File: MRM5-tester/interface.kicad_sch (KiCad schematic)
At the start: 28 parts, among them J1 Conn_01x02, J2 Conn_01x02, J3 GSB1C41110SSHR, J4 PINHD_1x2_Female, J5 PINHD_1x2_Female, J6 Conn_01x05, J7 Conn_01x05, Q5 SMMBT3906LT3G, Q6 SMMBT3906LT3G, U1 CP2102N-A02-GQFN20

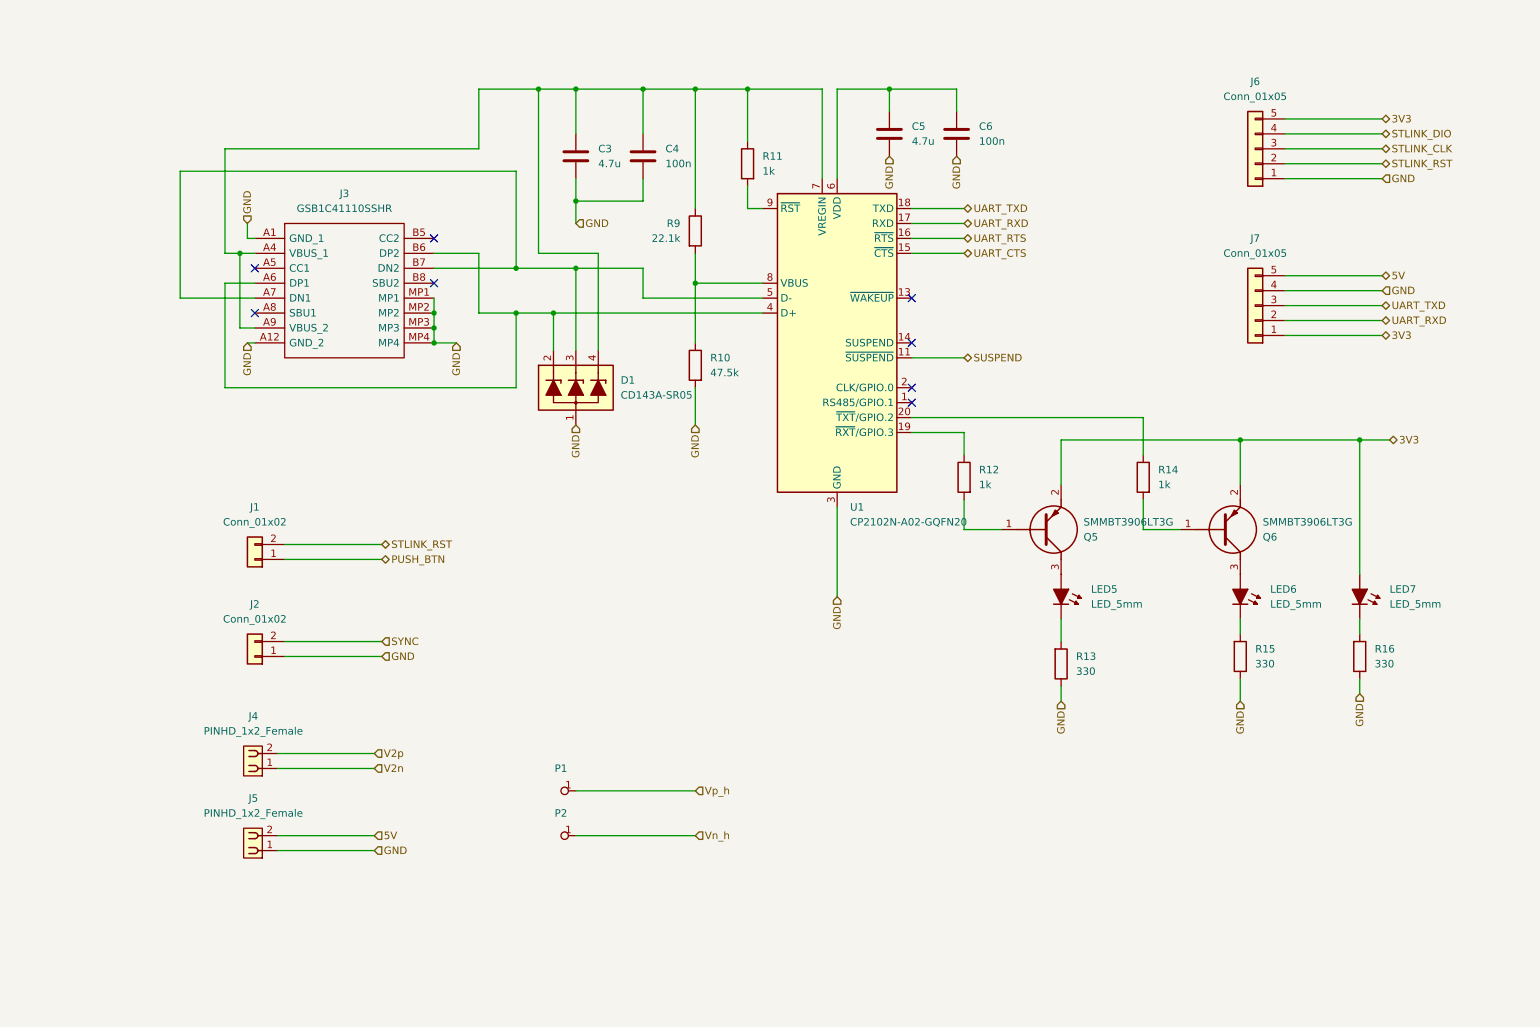
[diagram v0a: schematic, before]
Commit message: 케이스에 마춰서 제작 중
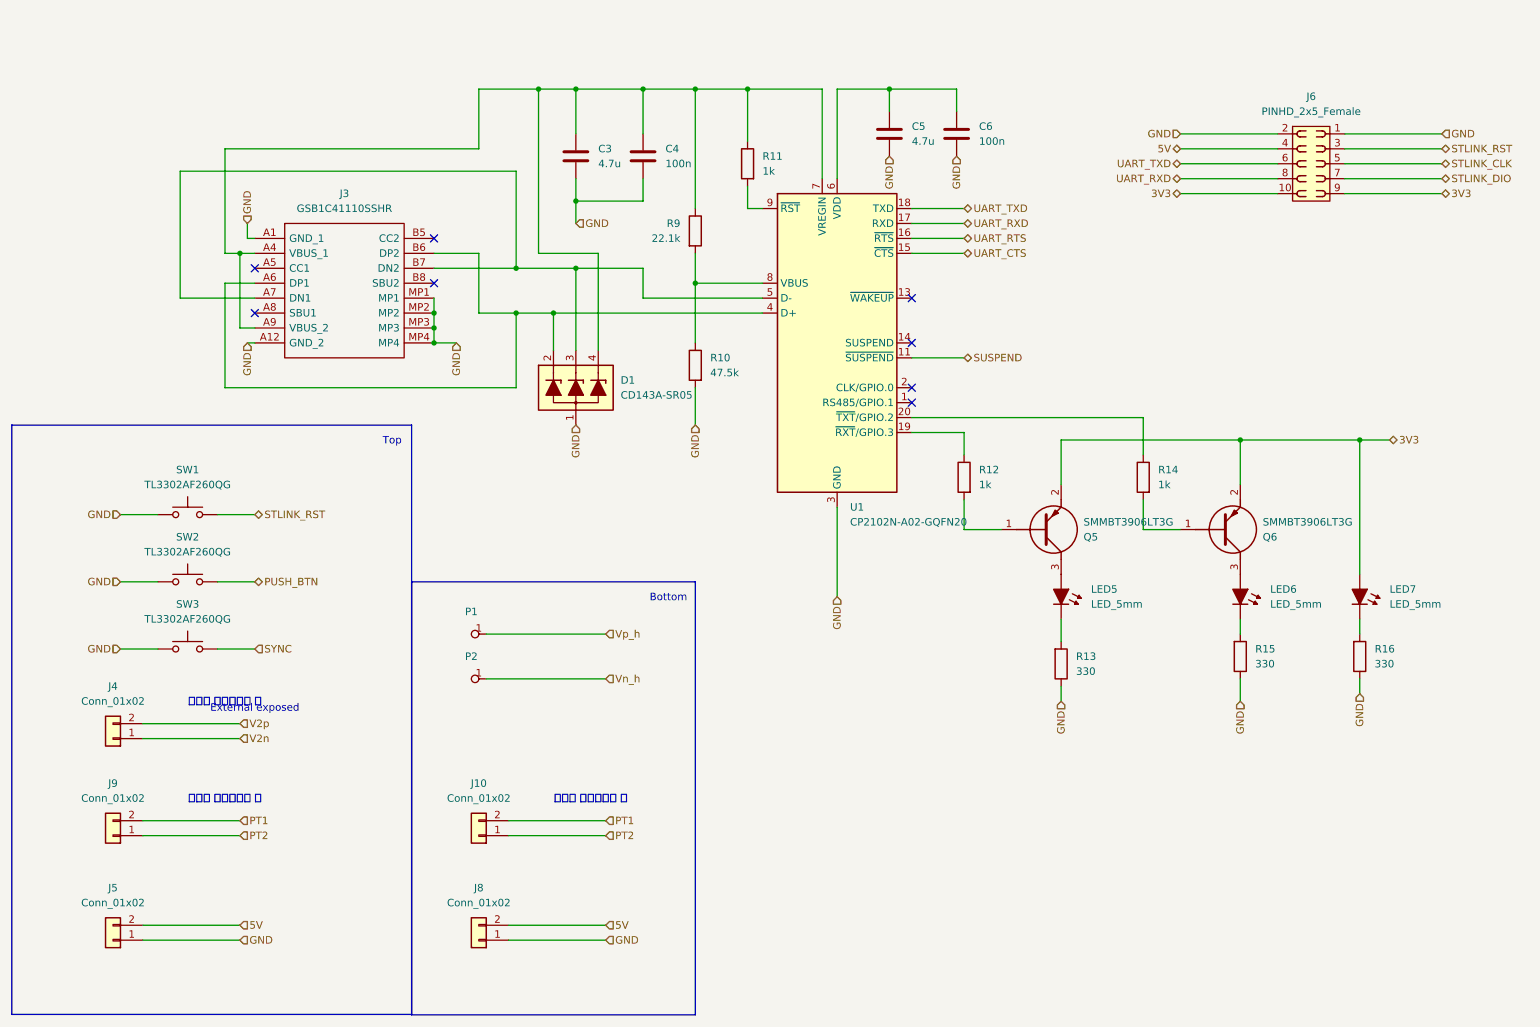
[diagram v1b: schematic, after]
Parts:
- removed J1, J2: Conn_01x02, Connector_PinHeader_2.54mm:PinHeader_1x02_P2.54mm_Vertical, symbol PCM_4ms_Connector:Conn_01x02
- removed J4, J5: PINHD_1x2_Female, Connector_PinSocket_2.54mm:PinSocket_1x02_P2.54mm_Vertical, symbol PCM_SL_Pin_Headers:PINHD_1x2_Female
- removed J6, J7: Conn_01x05, Connector_PinSocket_2.54mm:PinSocket_1x05_P2.54mm_Vertical, symbol Connector_Generic:Conn_01x05
- added J10, J4, J5, J8, J9: Conn_01x02, Connector_PinHeader_2.54mm:PinHeader_1x02_P2.54mm_Vertical, symbol PCM_4ms_Connector:Conn_01x02
- added J6: PINHD_2x5_Female, Connector_PinSocket_2.54mm:PinSocket_2x05_P2.54mm_Vertical, symbol PCM_SL_Pin_Headers:PINHD_2x5_Female
- added SW1, SW2, SW3: TL3302AF260QG, Mouser:TL3302AF260QG, symbol Switch:SW_Omron_B3FS
- LED5, LED6, LED7: footprint PCM_LED_THT_AKL:LED_D5.0mm -> PCM_LED_SMD_Handsoldering_AKL:LED_1206_3216Metric
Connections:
- net 3V3: now also J6.10, J6.9
- net 5V: now also J5.2 (Pin_2), J6.4, J8.2 (Pin_2)
- net GND: now also J5.1 (Pin_1), J6.1, J6.2, J8.1 (Pin_1), SW1.1, SW2.1, SW3.1
- net PUSH_BTN: now also SW2.2
- net STLINK_CLK: now also J6.5
- net STLINK_DIO: now also J6.7
- net STLINK_RST: now also J6.3, SW1.2
- net SYNC: now also SW3.2
- net UART_RXD: now also J6.8
- net UART_TXD: now also J6.6
- net V2n: now also J4.1 (Pin_1)
- net V2p: now also J4.2 (Pin_2)
- new net PT1: J10.2 (Pin_2), J9.2 (Pin_2)
- new net PT2: J10.1 (Pin_1), J9.1 (Pin_1)
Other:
- note added: "Bottom"
- note added: "External exposed"
- note added: "Top"
- note added: "외부로 노출되어야 함"
- moved on the sheet: P1, P2

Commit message: 1차 마감
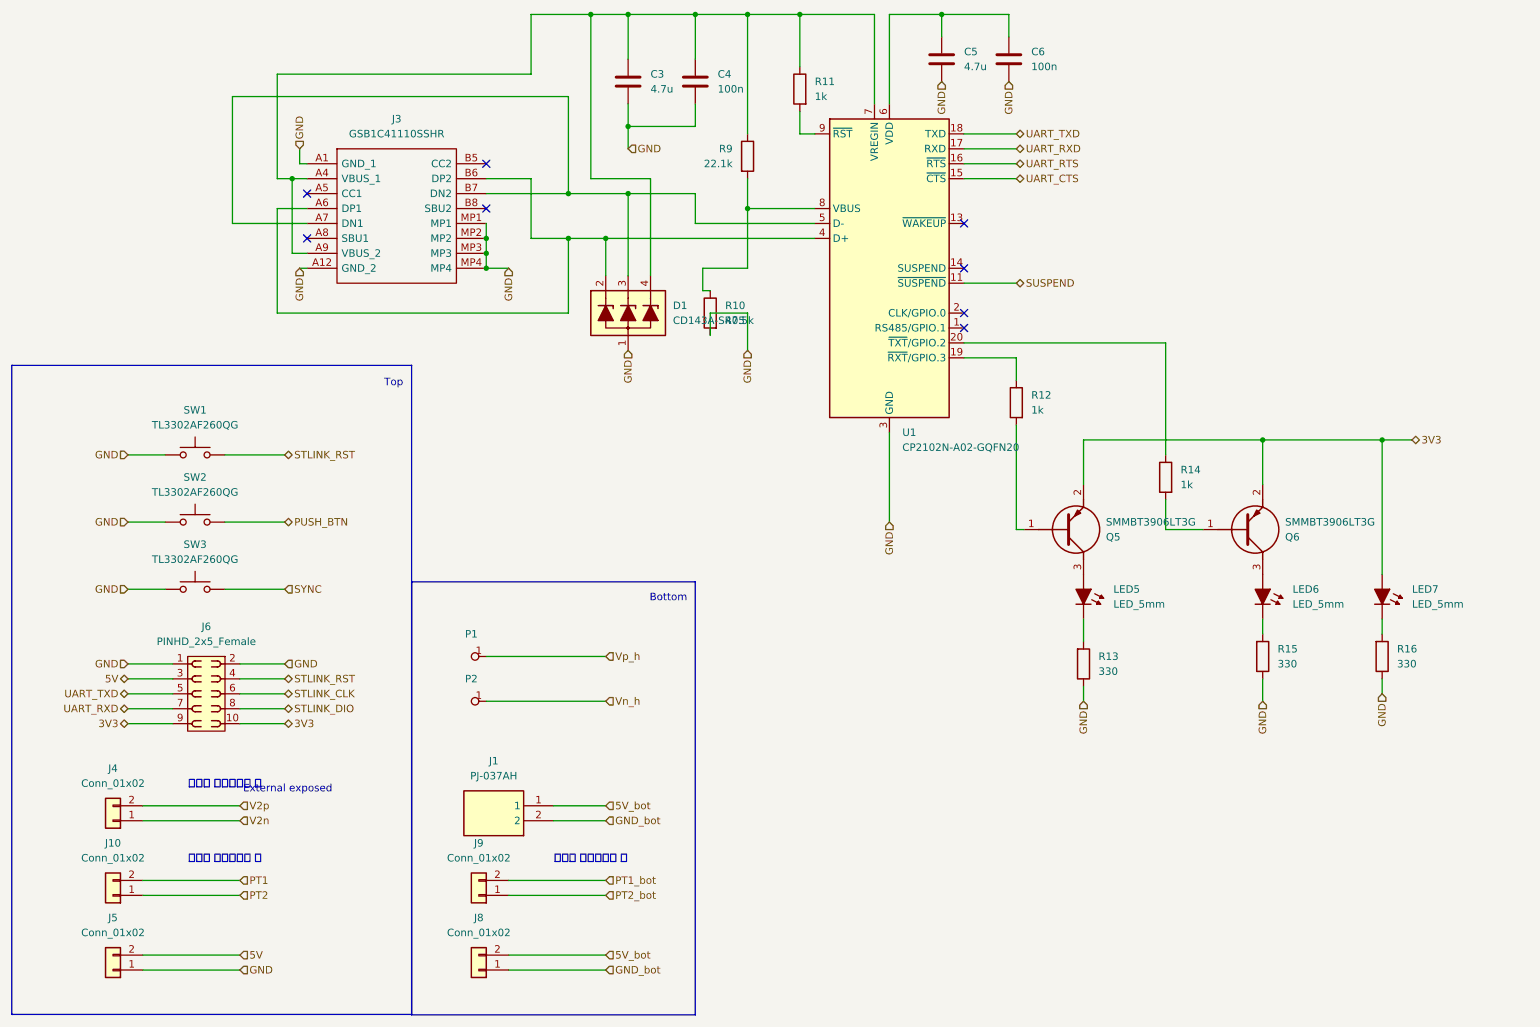
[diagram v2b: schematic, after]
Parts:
- added J1: PJ-037AH, PJ037AH, symbol Mouser:PJ-037AH
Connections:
- net 5V: now also J6.3; no longer J6.4, J8.2 (Pin_2)
- net GND: no longer J8.1 (Pin_1)
- net PT1: no longer J9.2 (Pin_2)
- net PT2: no longer J9.1 (Pin_1)
- net STLINK_CLK: now also J6.6; no longer J6.5
- net STLINK_DIO: now also J6.8; no longer J6.7
- net STLINK_RST: now also J6.4; no longer J6.3
- net UART_RXD: now also J6.7; no longer J6.8
- net UART_TXD: now also J6.5; no longer J6.6
- new net 5V_bot: J1.1, J8.2 (Pin_2)
- new net GND_bot: J1.2, J8.1 (Pin_1)
- new net PT1_bot: J9.2 (Pin_2)
- new net PT2_bot: J9.1 (Pin_1)
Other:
- moved on the sheet: C3, C4, C5, C6, D1, J10, J3, J4, J5, J6, J8, J9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

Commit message: PCB 제작 1차 마감
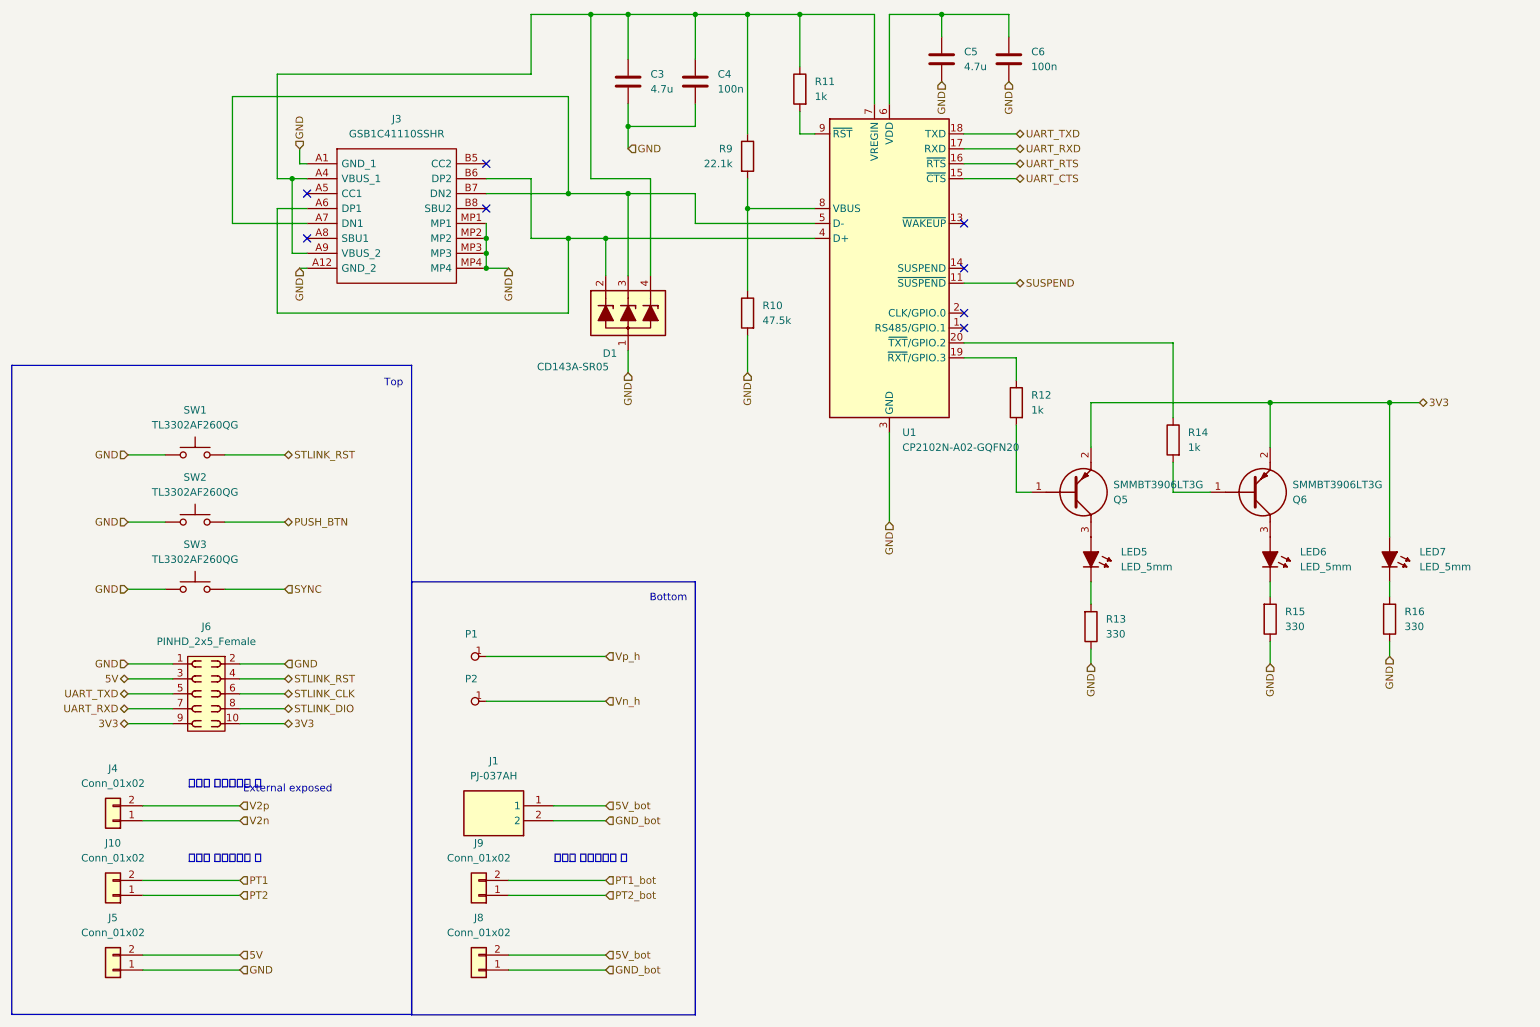
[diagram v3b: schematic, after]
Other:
- moved on the sheet: LED5, LED6, LED7, Q5, Q6, R10, R13, R14, R15, R16
